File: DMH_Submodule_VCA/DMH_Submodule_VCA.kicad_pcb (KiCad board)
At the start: 2 copper layers, 40 x 40 mm, 19 parts, among them J1 Conn_02x03_Odd_Even, Q1 BC548, Q2 BC548, U1 TL072

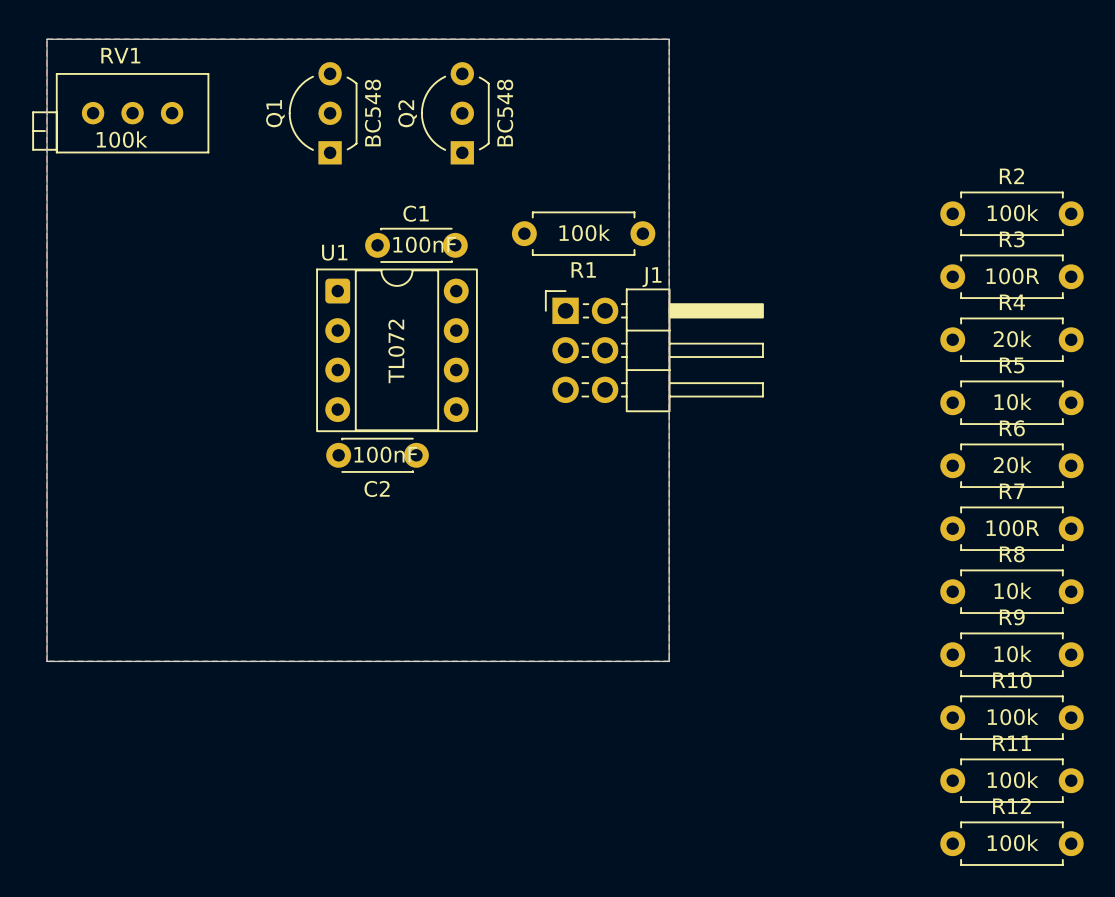
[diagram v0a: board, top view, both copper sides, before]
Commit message: Designed PCB
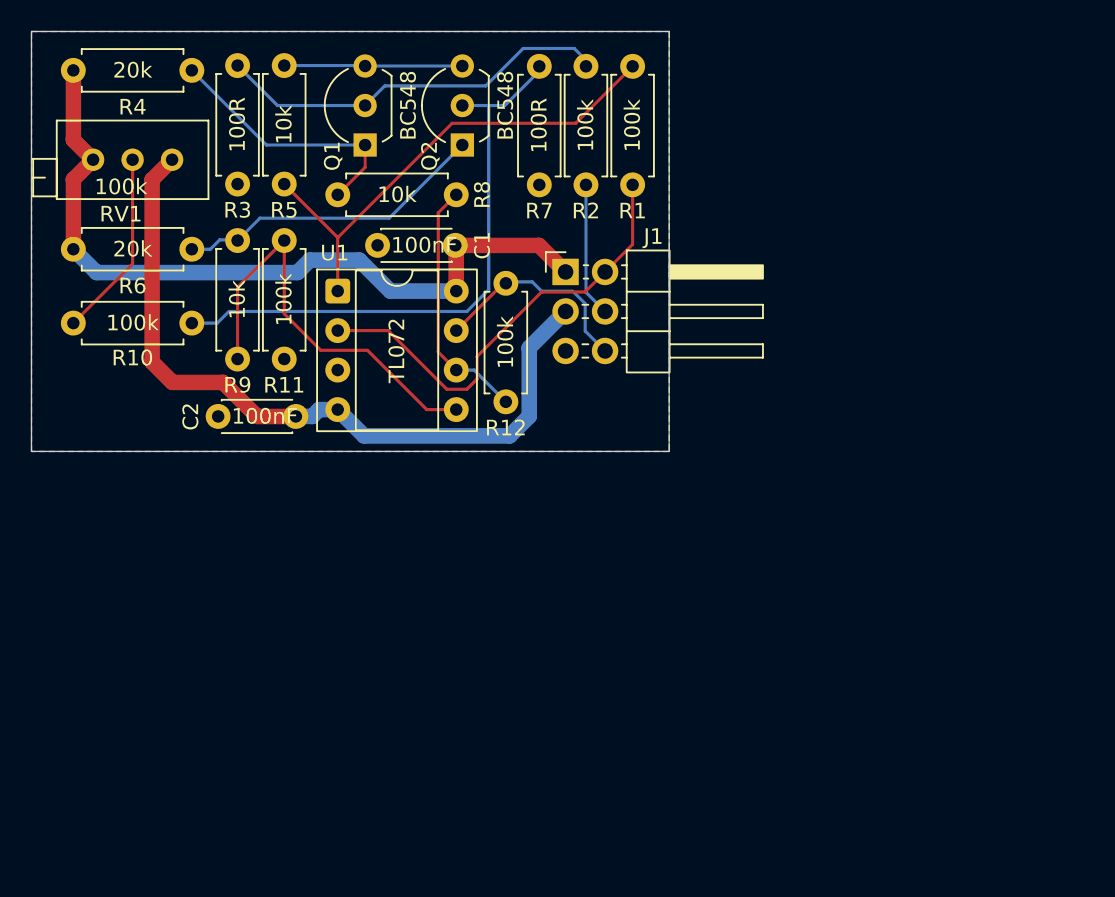
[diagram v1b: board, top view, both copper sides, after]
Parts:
- moved R10 62.0 mm to (56.7, 68.2)
- moved R11 55.3 mm to (70.2, 62.9), turned to -90 degrees
- moved R4 51.9 mm to (64.3, 52.0), turned to 180 degrees
- moved R6 50.9 mm to (64.3, 63.5), turned to 180 degrees
- moved R9 49.8 mm to (67.2, 70.6), turned to 90 degrees
- moved R3 46.4 mm to (67.2, 59.3), turned to 90 degrees
- moved R12 46.1 mm to (84.5, 65.7), turned to -90 degrees
- moved R5 45.2 mm to (70.2, 59.3), turned to 90 degrees
- moved R8 40.9 mm to (81.3, 60.0), turned to 180 degrees
- moved R7 34.6 mm to (86.7, 59.4), turned to 90 degrees
- moved R2 25.4 mm to (89.7, 51.7), turned to -90 degrees
- moved C2 13.0 mm to (66.0, 74.2), turned to 0 degrees
- moved R1 3.21 mm to (92.7, 59.4), turned to 90 degrees
- moved RV1 2.99 mm to (63.0, 57.7)
- moved J1 2.50 mm to (88.3, 65.0)
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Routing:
- net +12V: track 0.00 -> 49.7 mm
- net -12V: track 0.00 -> 48.4 mm
- net Net-(Q2-B): track 0.00 -> 38.2 mm
- net Net-(R1-Pad2): track 0.00 -> 31.9 mm
- net /CV Mix In: track 0.00 -> 29.1 mm
- net Net-(U1B-+): track 0.00 -> 27.2 mm
- net Net-(Q1-B): track 0.00 -> 25.8 mm
- net Net-(Q2-C): track 0.00 -> 20.2 mm
- net Net-(Q1-C): track 0.00 -> 17.1 mm
- net Net-(U1B--): track 0.00 -> 16.3 mm
- net /Signal Out: track 0.00 -> 13.7 mm
- net Net-(R10-Pad1): track 0.00 -> 12.1 mm
- net Net-(Q1-E): track 0.00 -> 11.5 mm
- net /Signal In: track 0.00 -> 8.65 mm
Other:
- board size 40 x 40 mm -> 41 x 27 mm
